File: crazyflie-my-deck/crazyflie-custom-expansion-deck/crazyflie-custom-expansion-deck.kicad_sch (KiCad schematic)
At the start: 5 parts, among them J1 Conn_01x10, J2 Conn_02x10_Odd_Even, J3 Conn_01x10

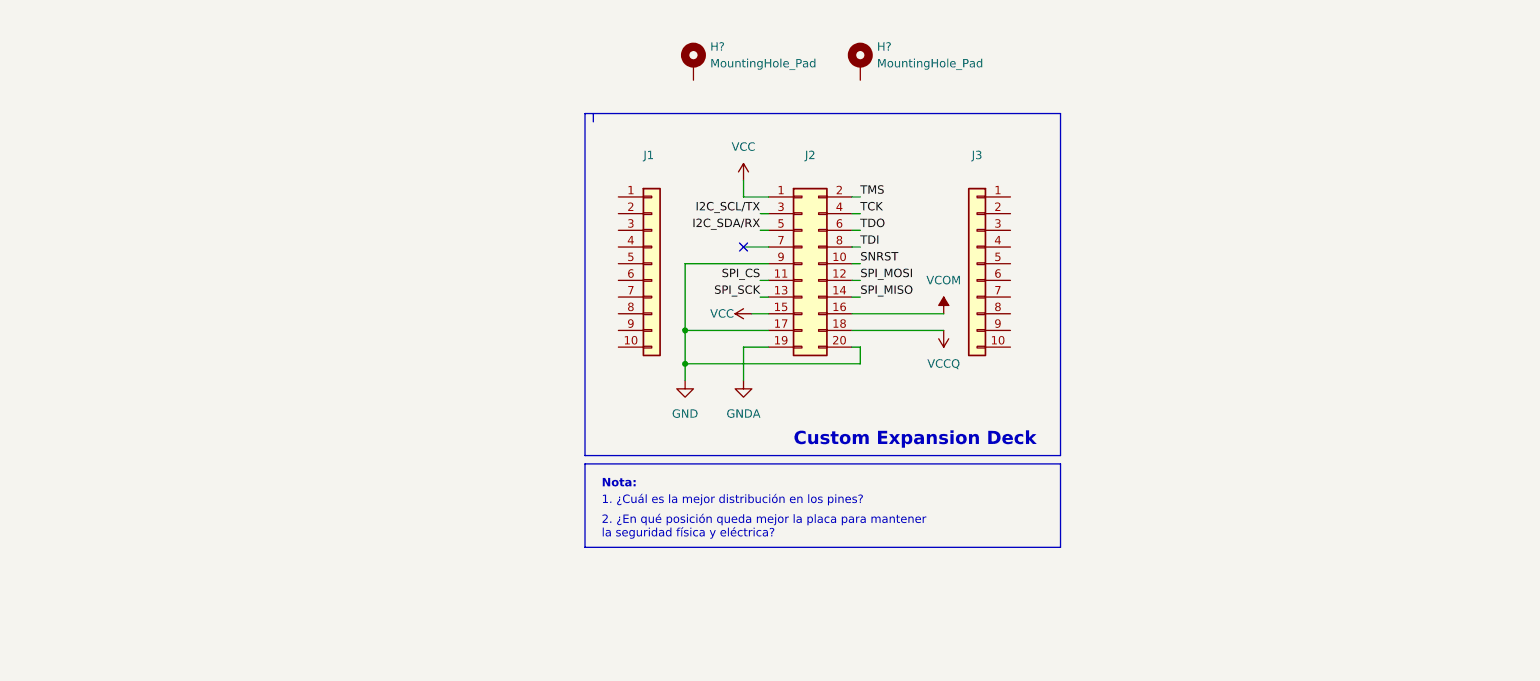
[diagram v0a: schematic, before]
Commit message: acomodo de componentes
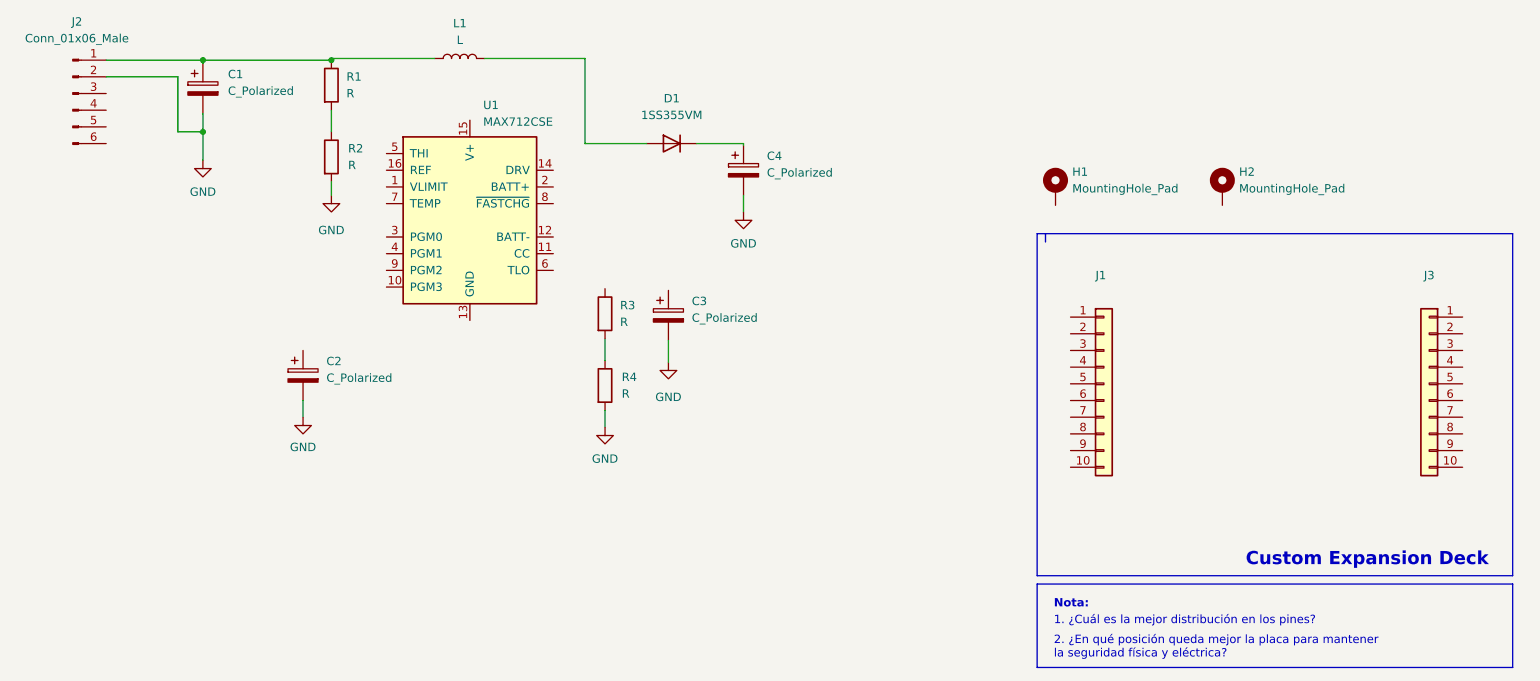
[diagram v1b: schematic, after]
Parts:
- removed J2: Conn_02x10_Odd_Even, Connector_PinHeader_1.27mm:PinHeader_2x10_P1.27mm_Vertical, symbol Connector_Generic:Conn_02x10_Odd_Even
- added C1, C4: C_Polarized, Capacitor_Tantalum_SMD:CP_EIA-3528-15_AVX-H, symbol Device:C_Polarized
- added C2: C_Polarized, Capacitor_SMD:C_0805_2012Metric, symbol Device:C_Polarized
- added C3: C_Polarized, Capacitor_SMD:C_1210_3225Metric, symbol Device:C_Polarized
- added D1: 1SS355VM, Diode_SMD:D_SOD-323F, symbol Diode:1SS355VM
- added J2: Conn_01x06_Male, Connector_PinHeader_1.27mm:PinHeader_1x06_P1.27mm_Horizontal, symbol Connector:Conn_01x06_Male
- added L1: L, Inductor_SMD:L_1210_3225Metric, symbol Device:L
- added R1, R2, R3, R4: R, Resistor_SMD:R_0805_2012Metric, symbol Device:R
- added U1: MAX712CSE, Package_SO:SOIC-16_3.9x9.9mm_P1.27mm, symbol Battery_Management:MAX712CSE
- gave numbers to parts that had none: 2
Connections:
- net GND: now also C1.2, C2.2, C3.2, C4.2, J2.2 (Pin_2), R2.2, R4.2
- new net: R3.2, R4.1
- new net: C1.1, J2.1 (Pin_1), L1.1, R1.1
- new net: D1.2 (A), L1.2
- new net: R1.2, R2.1
- new net: C4.1, D1.1 (K)
- no-connect marks 1 -> 0
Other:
- moved on the sheet: H1, H2, J1, J3
